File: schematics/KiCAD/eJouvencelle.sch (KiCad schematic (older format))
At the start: 42 parts

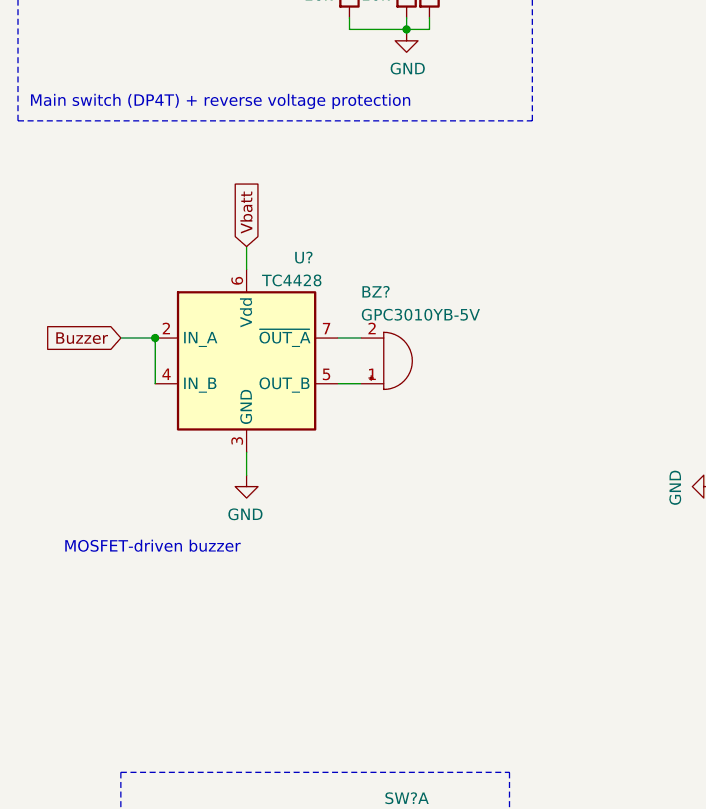
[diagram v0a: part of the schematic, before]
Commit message: Update eJouvencelle.sch
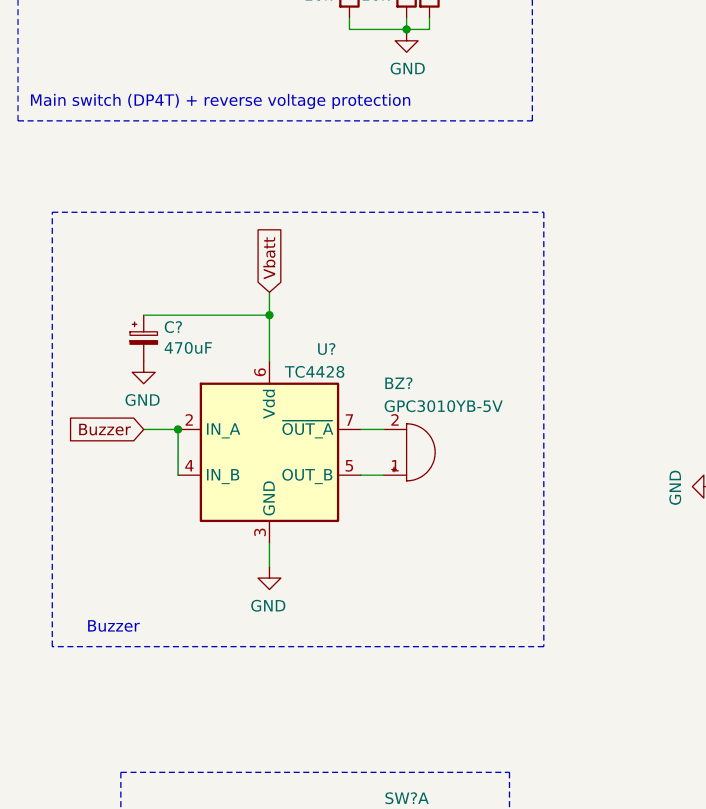
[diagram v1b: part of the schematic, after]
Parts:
- added C?: 470uF, symbol Device:CP_Small
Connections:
- net GND: now also C?.2
- net Vbatt: now also C?.1
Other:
- note added: "Buzzer"
- note removed: "MOSFET-driven buzzer"
- moved on the sheet: BZ?, U?
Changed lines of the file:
@@
 Text Notes 7800 3100 0    50   ~ 0
 7-segment w/ BCD decoder
-Text GLabel 2000 3250 1    50   Input ~ 0
+Text GLabel 2100 3450 1    50   Input ~ 0
 Vbatt
-Text GLabel 1450 3650 0    50   Input ~ 0
+Text GLabel 1550 4050 0    50   Input ~ 0
 Buzzer
-Text Notes 1200 4600 0    50   ~ 0
-MOSFET-driven buzzer
+Text Notes 1300 4950 0    50   ~ 0
+Buzzer
 Text GLabel 4550 5150 0    50   Input ~ 0
 Buzzer
@@
 L power:GND #PWR?
 U 1 1 5EA2FE7F
-P 2000 4250
-F 0 "#PWR?" H 2000 4000 50  0001 C CNN
-F 1 "GND" H 2005 4077 50  0000 C CNN
-F 2 "" H 2000 4250 50  0001 C CNN
-F 3 "" H 2000 4250 50  0001 C CNN
-	1    2000 4250
+P 2100 4650
+F 0 "#PWR?" H 2100 4400 50  0001 C CNN
+F 1 "GND" H 2105 4477 50  0000 C CNN
+F 2 "" H 2100 4650 50  0001 C CNN
+F 3 "" H 2100 4650 50  0001 C CNN
+	1    2100 4650
 	-1   0    0    -1
 $EndComp
@@
 L Device:Buzzer BZ?
 U 1 1 5E9C10D5
-P 2600 3750
-F 0 "BZ?" H 2500 3450 50  0000 L CNN
-F 1 "GPC3010YB-5V" H 2500 3550 50  0000 L CNN
-F 2 "" V 2575 3850 50  0001 C CNN
-F 3 "~" V 2575 3850 50  0001 C CNN
-	1    2600 3750
+P 2700 4150
+F 0 "BZ?" H 2600 3850 50  0000 L CNN
+F 1 "GPC3010YB-5V" H 2600 3950 50  0000 L CNN
+F 2 "" V 2675 4250 50  0001 C CNN
+F 3 "~" V 2675 4250 50  0001 C CNN
+	1    2700 4150
 	1    0    0    1
 $EndComp
@@
 Wire Wire Line
 	5100 2800 5100 2850
+Wire Wire Line
+	1700 4050 1700 4250
+Wire Wire Line
+	1550 4050 1700 4050
+Wire Wire Line
+	2500 4050 2600 4050
+Wire Wire Line
+	2500 4250 2600 4250
+Wire Wire Line
+	2100 4550 2100 4650
+$Comp
+L power:GND #PWR?
+U 1 1 60E9B367
+P 1550 3750
+F 0 "#PWR?" H 1550 3500 50  0001 C CNN
+F 1 "GND" H 1555 3577 50  0000 C CNN
+F 2 "" H 1550 3750 50  0001 C CNN
+F 3 "" H 1550 3750 50  0001 C CNN
+	1    1550 3750
+	-1   0    0    -1
+$EndComp
+Wire Wire Line
+	2100 3450 2100 3550
+Connection ~ 2100 3550
+Wire Wire Line
+	2100 3550 2100 3750
+Connection ~ 1700 4050
 $Comp
 L eJouvencelle:TC4428 U?
 U 1 1 60E78FEB
-P 2000 3750
-F 0 "U?" H 2250 4200 50  0000 C CNN
-F 1 "TC4428" H 2200 4100 50  0000 C CNN
-F 2 "Package_SO:MSOP-8_3x3mm_P0.65mm" H 1950 3250 50  0001 C CNN
-F 3 "http://ww1.microchip.com/downloads/en/devicedoc/hv9967b.pdf" H 2000 3750 50  0001 C CNN
-	1    2000 3750
-	1    0    0    -1
-$EndComp
-Wire Wire Line
-	1600 3650 1600 3850
-Wire Wire Line
-	1450 3650 1600 3650
-Connection ~ 1600 3650
-Wire Wire Line
-	2400 3650 2500 3650
-Wire Wire Line
-	2400 3850 2500 3850
-Wire Wire Line
-	2000 3250 2000 3350
-Wire Wire Line
-	2000 4150 2000 4250
+P 2100 4150
+F 0 "U?" H 2350 4600 50  0000 C CNN
+F 1 "TC4428" H 2300 4500 50  0000 C CNN
+F 2 "Package_SO:MSOP-8_3x3mm_P0.65mm" H 2050 3650 50  0001 C CNN
+F 3 "http://ww1.microchip.com/downloads/en/devicedoc/hv9967b.pdf" H 2100 4150 50  0001 C CNN
+	1    2100 4150
+	1    0    0    -1
+$EndComp
+$Comp
+L Device:CP_Small C?
+U 1 1 60E925D2
+P 1550 3650
+F 0 "C?" H 1638 3696 50  0000 L CNN
+F 1 "470uF" H 1638 3605 50  0000 L CNN
+F 2 "" H 1550 3650 50  0001 C CNN
+F 3 "~" H 1550 3650 50  0001 C CNN
+	1    1550 3650
+	1    0    0    -1
+$EndComp
+Wire Wire Line
+	1550 3550 2100 3550
+Wire Notes Line
+	1150 3100 3300 3100
+Wire Notes Line
+	3300 3100 3300 5000
+Wire Notes Line
+	3300 5000 1150 5000
+Wire Notes Line
+	1150 5000 1150 3100
 $EndSCHEMATC
